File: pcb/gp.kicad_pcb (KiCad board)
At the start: 2 copper layers, 52.1 x 20.3 mm, 33 parts, among them J1 USB_C_Receptacle_USB2.0, U1 XC6206P332MR, U2 STM32F103CBT6, Y1 8M, Y2 NM (32.768k)

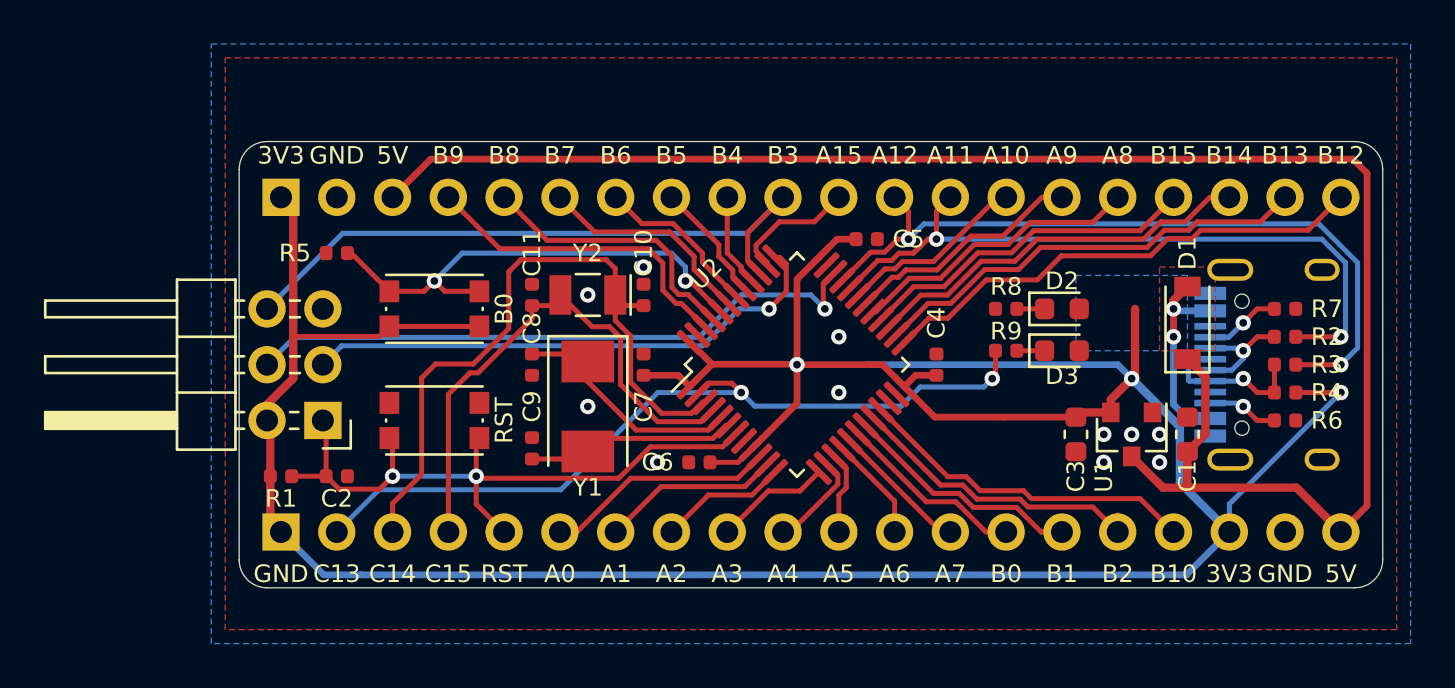
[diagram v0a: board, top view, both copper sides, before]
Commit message: Hmmm
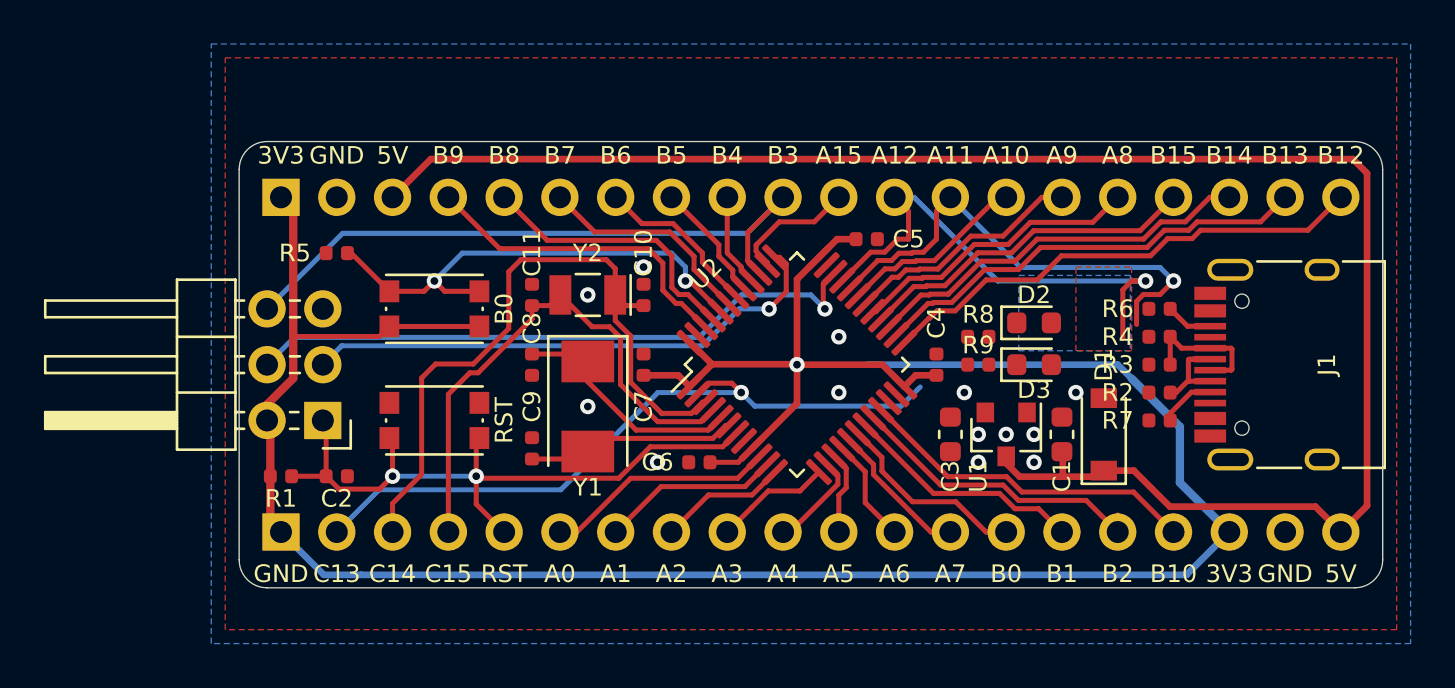
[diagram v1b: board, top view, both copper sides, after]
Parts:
- J1: moved to F.Cu
- moved R6 7.65 mm to (193.7, 99.1), turned to 180 degrees
- moved R7 7.65 mm to (193.7, 104.1), turned to 180 degrees
- moved D1 6.35 mm to (191.1, 104.8)
- moved R2 6.25 mm to (193.7, 102.9), turned to 180 degrees
- moved R4 6.25 mm to (193.7, 100.3), turned to 180 degrees
- moved C1 5.72 mm to (189.2, 104.8)
- moved C3 5.72 mm to (184.2, 104.8)
- moved U1 5.72 mm to (186.7, 104.8)
- moved R3 5.71 mm to (193.7, 101.6), turned to 180 degrees
- moved R8 1.80 mm to (185.4, 100.3)
- moved R9 1.42 mm to (185.4, 101.6)
- moved D2 1.42 mm to (188.0, 99.7)
- moved D3 1.42 mm to (188.0, 101.6)
- turned J1 to 90 degrees
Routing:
- net +3V3: track 146.8 -> 121.0 mm, vias 3 -> 2
- net A12: track 35.1 -> 23.0 mm, vias 2 -> 1
- net VBUS: track 10.5 -> 0.00 mm, vias 2 -> 0
- net A11: track 32.0 -> 22.2 mm, vias 2 -> 1
- net C13: track 37.0 -> 32.2 mm
- net Net-(D3-Pad1): track 1.27 -> 0.00 mm
- net Net-(D2-Pad1): track 1.27 -> 0.00 mm
- net Net-(J1-PadA6): track 7.44 -> 6.24 mm, vias 1 -> 0
- net Net-(J1-PadB5): track 3.25 -> 2.15 mm, vias 1 -> 0
- net Net-(J1-PadA5): track 3.46 -> 2.54 mm, vias 1 -> 0
- net +5V: track 79.7 -> 80.5 mm
- net Net-(J1-PadA7): track 5.32 -> 4.80 mm, vias 1 -> 0

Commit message: Rev c ready to order - production files gp_c verified.
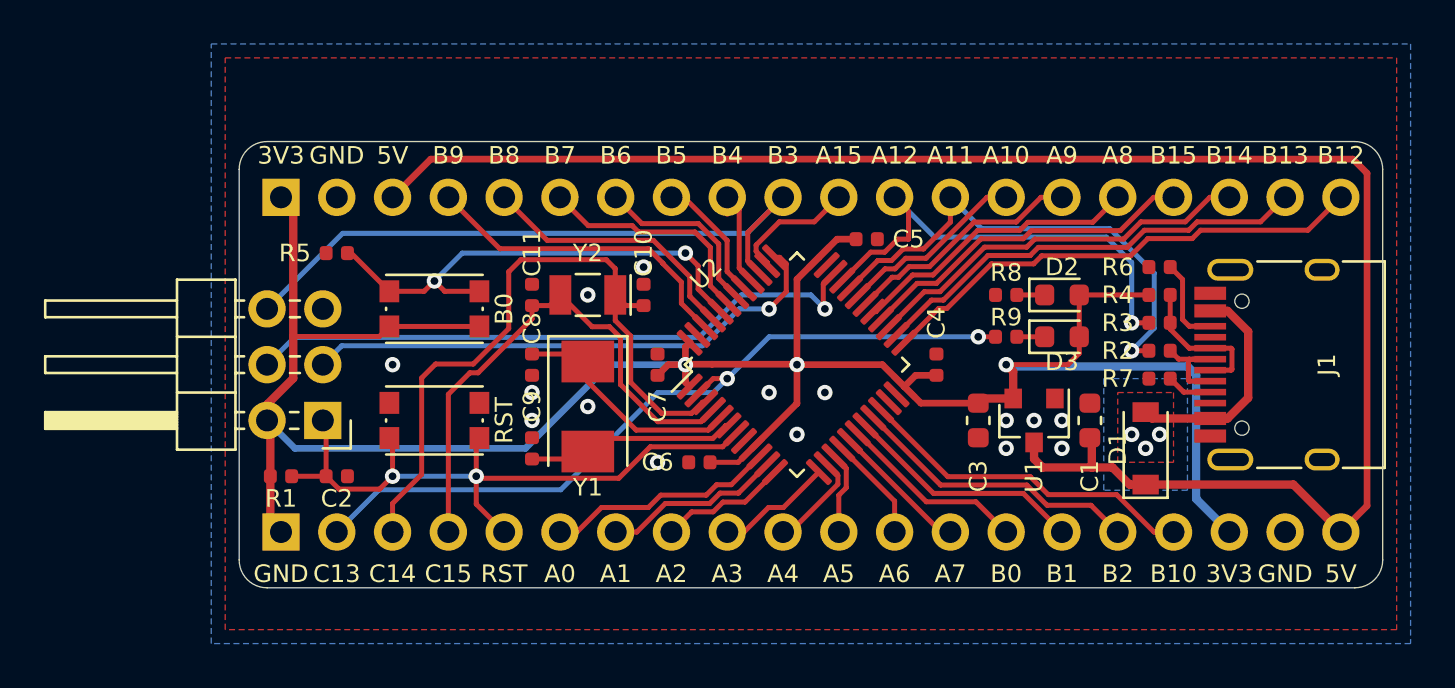
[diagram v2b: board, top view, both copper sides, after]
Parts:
- moved R8 2.29 mm to (186.7, 98.4)
- moved D1 2.01 mm to (193.0, 105.4)
- moved R2 1.91 mm to (193.7, 101.0)
- moved R3 1.91 mm to (193.7, 99.7)
- moved R4 1.91 mm to (193.7, 98.4)
- moved R6 1.91 mm to (193.7, 97.2)
- moved R7 1.91 mm to (193.7, 102.2)
- moved R9 1.80 mm to (186.7, 100.3)
- moved D2 1.80 mm to (189.2, 98.4)
- moved D3 1.80 mm to (189.2, 100.3)
- moved C1 1.42 mm to (190.5, 104.1)
- moved U1 1.42 mm to (188.0, 104.1)
- moved C3 1.42 mm to (185.4, 104.1)
- moved C7 0.63 mm to (170.8, 101.6)
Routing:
- net +3V3: track 121.0 -> 109.0 mm, vias 2 -> 3
- net VBUS: track 0.00 -> 10.3 mm, vias 0 -> 3
- net C13: track 32.2 -> 35.3 mm
- net Net-(J1-PadB5): track 2.15 -> 4.01 mm
- net Net-(D3-Pad1): track 0.00 -> 1.27 mm
- net Net-(D2-Pad1): track 0.00 -> 1.27 mm
- net A12: track 23.0 -> 22.2 mm
- net +5V: track 80.5 -> 79.7 mm
- net B7: track 10.0 -> 10.7 mm
- net B6: track 7.60 -> 8.28 mm
- net A11: track 22.2 -> 22.8 mm
- net GND: vias 11 -> 15

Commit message: Order rev c
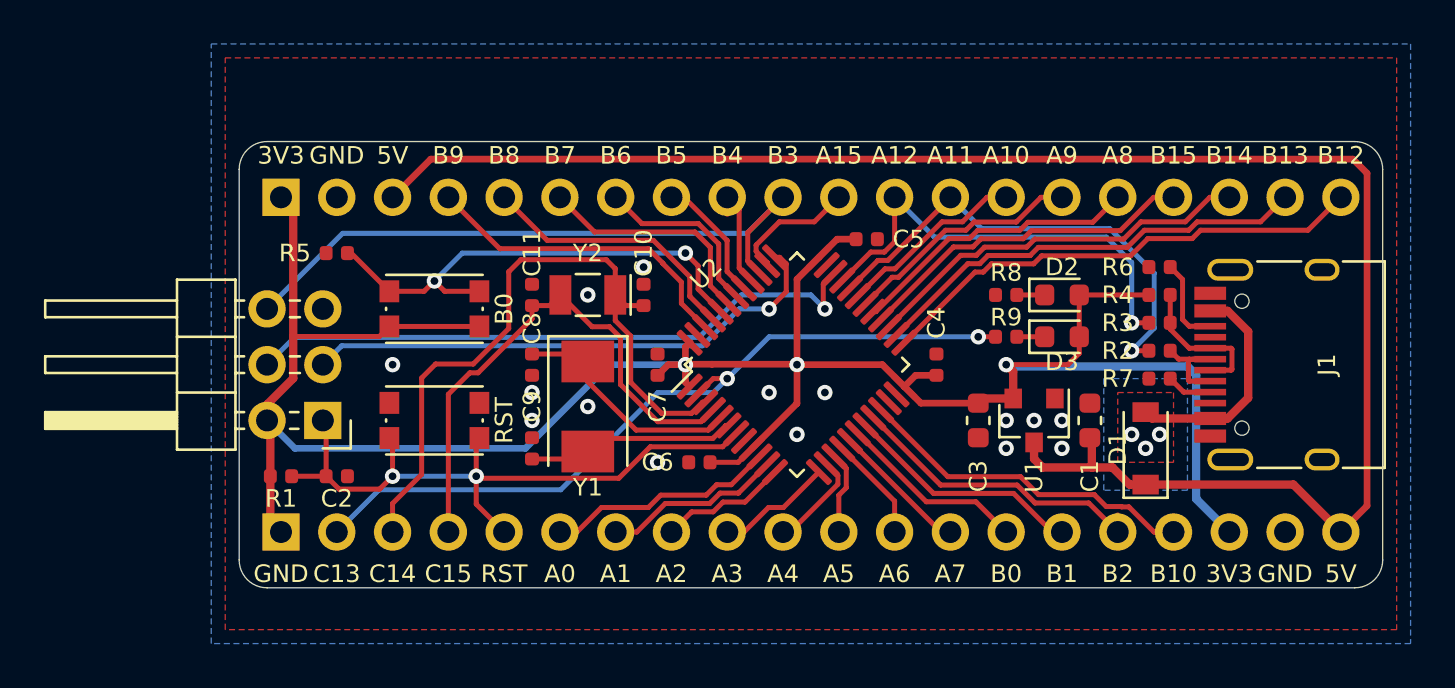
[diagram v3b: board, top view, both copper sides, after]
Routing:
- net A12: track 22.2 -> 21.3 mm
- net A11: track 22.8 -> 22.1 mm
